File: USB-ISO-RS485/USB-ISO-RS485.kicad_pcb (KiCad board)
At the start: 2 copper layers, 94.5 x 27.4 mm, 37 parts, among them P1 RS485 Connector, P10 TST, P11 TST, P12 TST, P13 UART Interface, P2 USB_A, P3 TST, P4 TST, P5 TST, P6 TST, P7 TST, P8 TST, P9 TST, U1 ADM2582E, U2 FT232RL

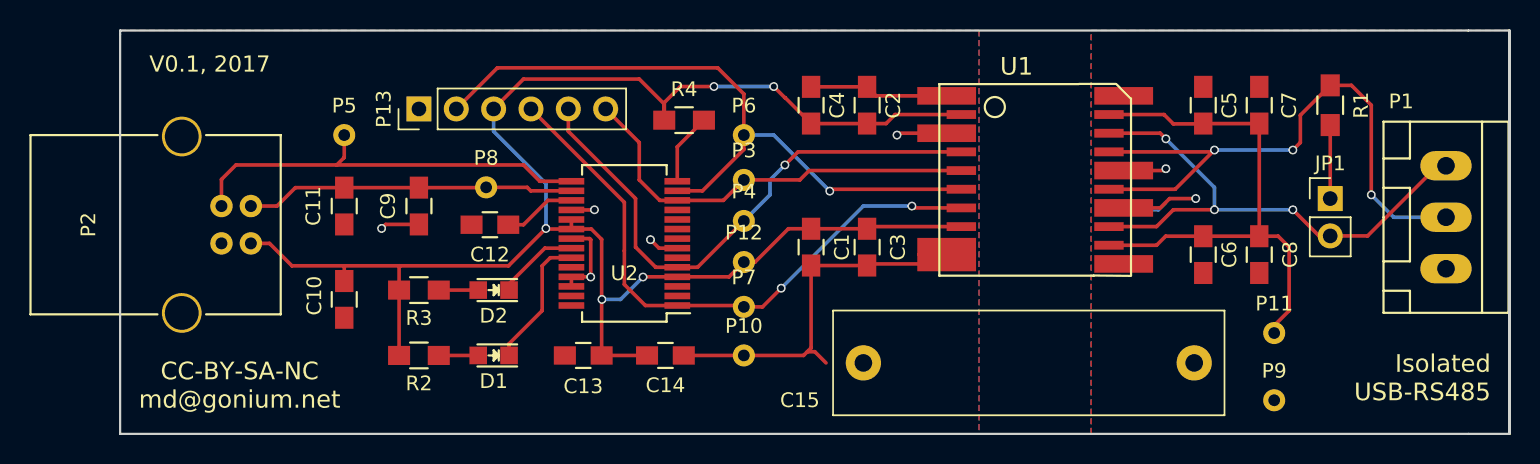
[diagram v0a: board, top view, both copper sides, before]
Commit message: v0.2 board layout complete
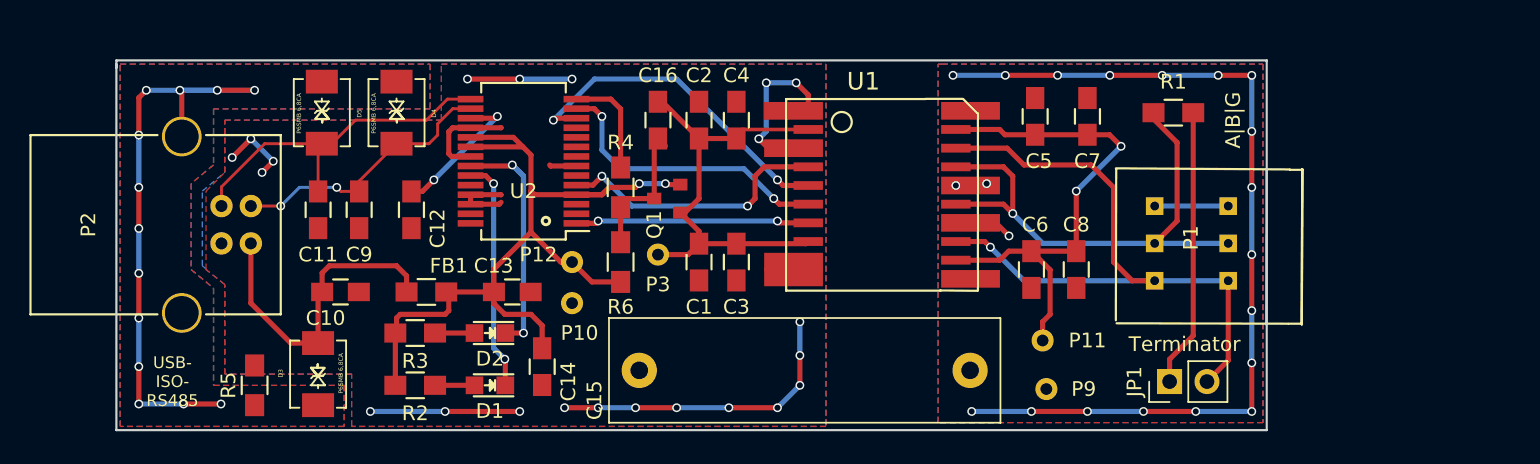
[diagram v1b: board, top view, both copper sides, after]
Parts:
- removed P13: UART Interface, Pin_Headers:Pin_Header_Straight_1x06_Pitch2.54mm
- removed P4, P5, P6, P7, P8: TST, Measurement_Points:Measurement_Point_Round-TH_Small
- added C16: 100nF, Capacitors_SMD:C_0805_HandSoldering, F.Cu at (122.9, 70.4)
- added D3: P6SMB 6,8CA, ADM2582E:P6SMB6,8CA, F.Cu at (99.8, 87.6)
- added D4: P6SMB 6,8CA, ADM2582E:P6SMB6,8CA, F.Cu at (105.2, 69.8)
- added D5: P6SMB 6,8CA, ADM2582E:P6SMB6,8CA, F.Cu at (100.1, 69.8)
- added FB1: BLM21PG 600, Resistors_SMD:R_0805_HandSoldering, F.Cu at (107.2, 82.0)
- added Q1: IRLML6402, ADM2582E:IRLML6402, F.Cu at (122.7, 75.7)
- added R5: 0, Resistors_SMD:R_0805_HandSoldering, F.Cu at (95.5, 88.4)
- added R6: 100k, Resistors_SMD:R_0805_HandSoldering, F.Cu at (120.4, 80.0)
- P1: value RS485 Connector -> WAGO 233-503; footprint Connectors_WAGO:WAGO_734_3pin_Straight_RuggedPads -> ADM2582E:WAGO233-503
- R4: value 10k -> 4k7
- moved P1 20.3 mm to (156.7, 81.3), turned to 90 degrees
- moved JP1 16.6 mm to (157.7, 88.1), turned to 90 degrees
- moved P11 15.8 mm to (149.1, 85.3)
- moved P9 15.5 mm to (149.4, 88.6)
- moved C15 15.2 mm to (121.7, 87.4)
- moved C8 12.5 mm to (151.4, 80.5)
- moved P10 12.2 mm to (117.1, 82.8)
- moved C6 11.7 mm to (148.3, 80.5)
- moved C7 11.7 mm to (152.1, 70.1)
- moved P12 11.7 mm to (117.1, 80.0)
- moved C2 11.5 mm to (125.7, 70.4)
- moved C5 11.5 mm to (148.6, 70.1)
- moved R1 10.7 mm to (158.0, 69.8), turned to 0 degrees
- moved U1 10.5 mm to (131.8, 69.1)
- moved C3 8.95 mm to (128.3, 80.0)
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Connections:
- C1 pad 1: +5V -> 5V-Switched
- C10 pad 1: +5V -> Net-(C10-Pad1)
- C11 pad 1: GND -> USBD+
- C11 pad 2: USBD- -> GND
- C2 pad 1: +5V -> 5V-Switched
- C3 pad 1: +5V -> 5V-Switched
- C4 pad 1: +5V -> 5V-Switched
- C9 pad 1: GND -> USBD-
- C9 pad 2: USBD- -> GND
- P2 pad 1: +5V -> Net-(C10-Pad1)
- P2 pad 5: GND -> Shield
- P3 pad 1: ~RE -> 5V-Switched
- R4 pad 1: +5V -> Net-(R4-Pad1)
- R4 pad 2: Net-(R4-Pad2) -> Net-(C16-Pad2)
- U1 pad 2: +5V -> 5V-Switched
- U1 pad 8: +5V -> 5V-Switched
- U2 pad 14: Net-(R4-Pad2) -> Net-(R4-Pad1)
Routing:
- net GNDA: track 10.1 -> 75.5 mm, vias 2 -> 21
- net +5V: track 117.8 -> 58.2 mm, vias 5 -> 2
- net Shield: track 0.00 -> 42.8 mm, vias 0 -> 13
- net (no net): track 1.73 -> 43.3 mm, vias 0 -> 19
- net 5V-Switched: track 0.00 -> 30.8 mm
- net GND: track 52.9 -> 25.4 mm, vias 5 -> 3
- net DE: track 47.1 -> 19.8 mm, vias 1 -> 2
- net TxD: track 41.0 -> 15.9 mm
- net Net-(C10-Pad1): track 0.00 -> 22.0 mm
- net RxD: track 37.6 -> 18.9 mm, vias 1 -> 2
- net Net-(JP1-Pad1): track 5.00 -> 19.0 mm
- net Net-(D2-Pad1): track 5.66 -> 16.9 mm, vias 0 -> 2
- net A: track 36.3 -> 47.3 mm, vias 3 -> 2
- net Net-(C16-Pad2): track 0.00 -> 9.61 mm
- net Net-(R4-Pad1): track 0.00 -> 7.27 mm
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- added copper zone on B.Cu, net Shield
- added copper zone on F.Cu, net Shield
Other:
- board size 94.5 x 27.4 mm -> 78.2 x 25.1 mm
- net class Data added: clearance 0.2, trace_width 0.2, via_dia 0.6, via_drill 0.4
- net class Default: trace_width 0.25 -> 0.35
- board text added: "A|B|G"
- board text added: "Connection: A, B and GND Terminator: 120 Ohm"
- board text added: "Isolated USB-RS485 Adaptor v0.2, 2017 CC-BY-NC-SA md@gonium.net"
- board text added: "Terminator"
- board text added: "USB- ISO- RS485"
- board text removed: "CC-BY-SA-NC md@gonium.net"
- board text removed: "Isolated USB-RS485"
- board text removed: "V0.1, 2017"
